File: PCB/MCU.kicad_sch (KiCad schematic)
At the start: 46 parts, among them J2 Conn_01x05_Pin, J3 Conn_01x02_Pin, SW1 SKRKAHE020, U1 STM32WLE5CCUx, U7 STM32WLE5C8Ux, Y1 ECS-TXO-25CSMV

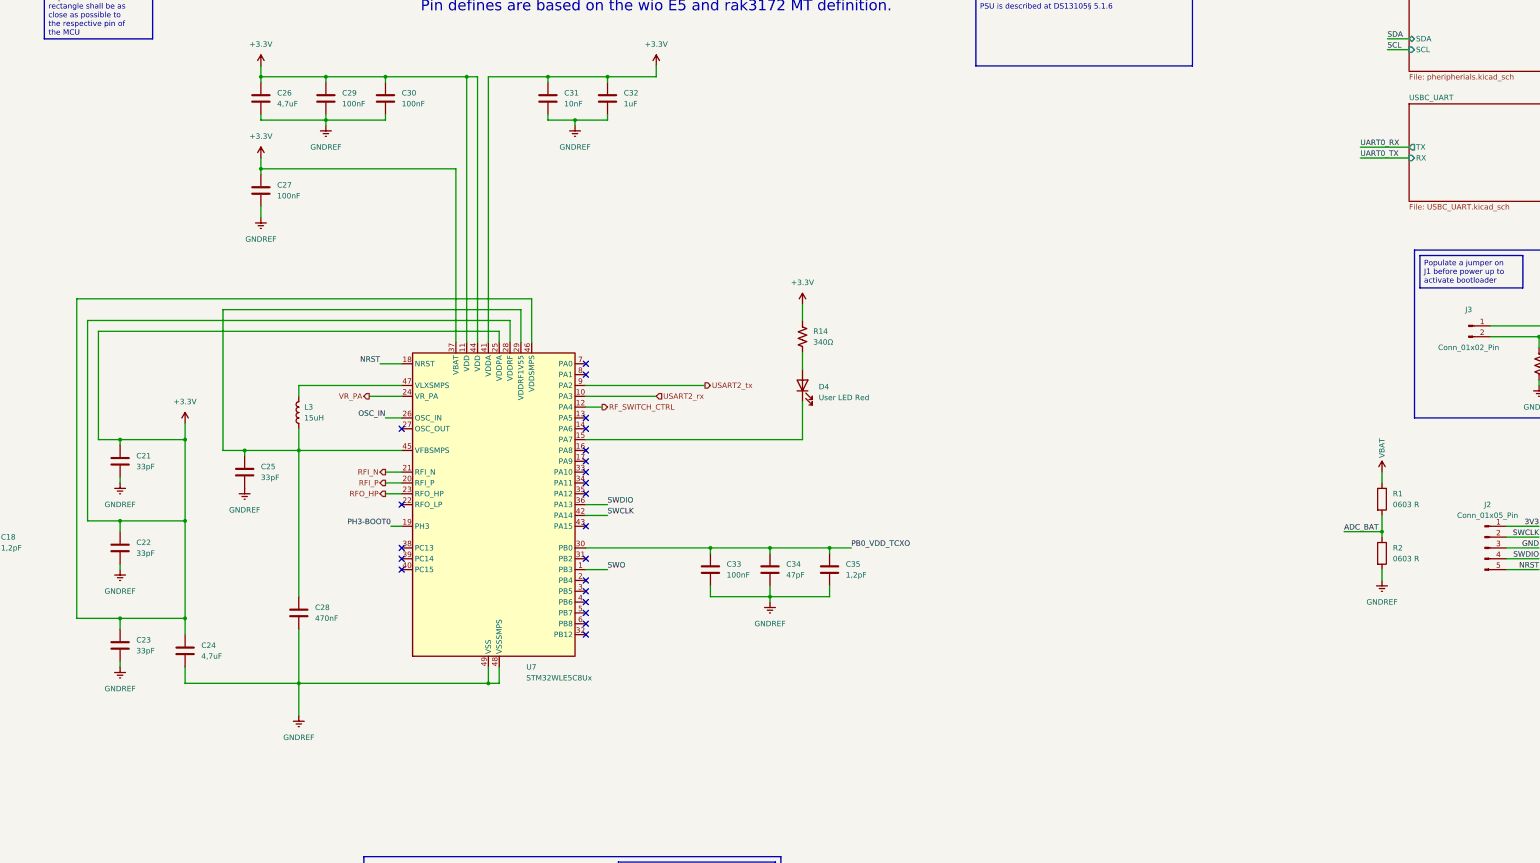
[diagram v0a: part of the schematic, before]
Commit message: finished the migration
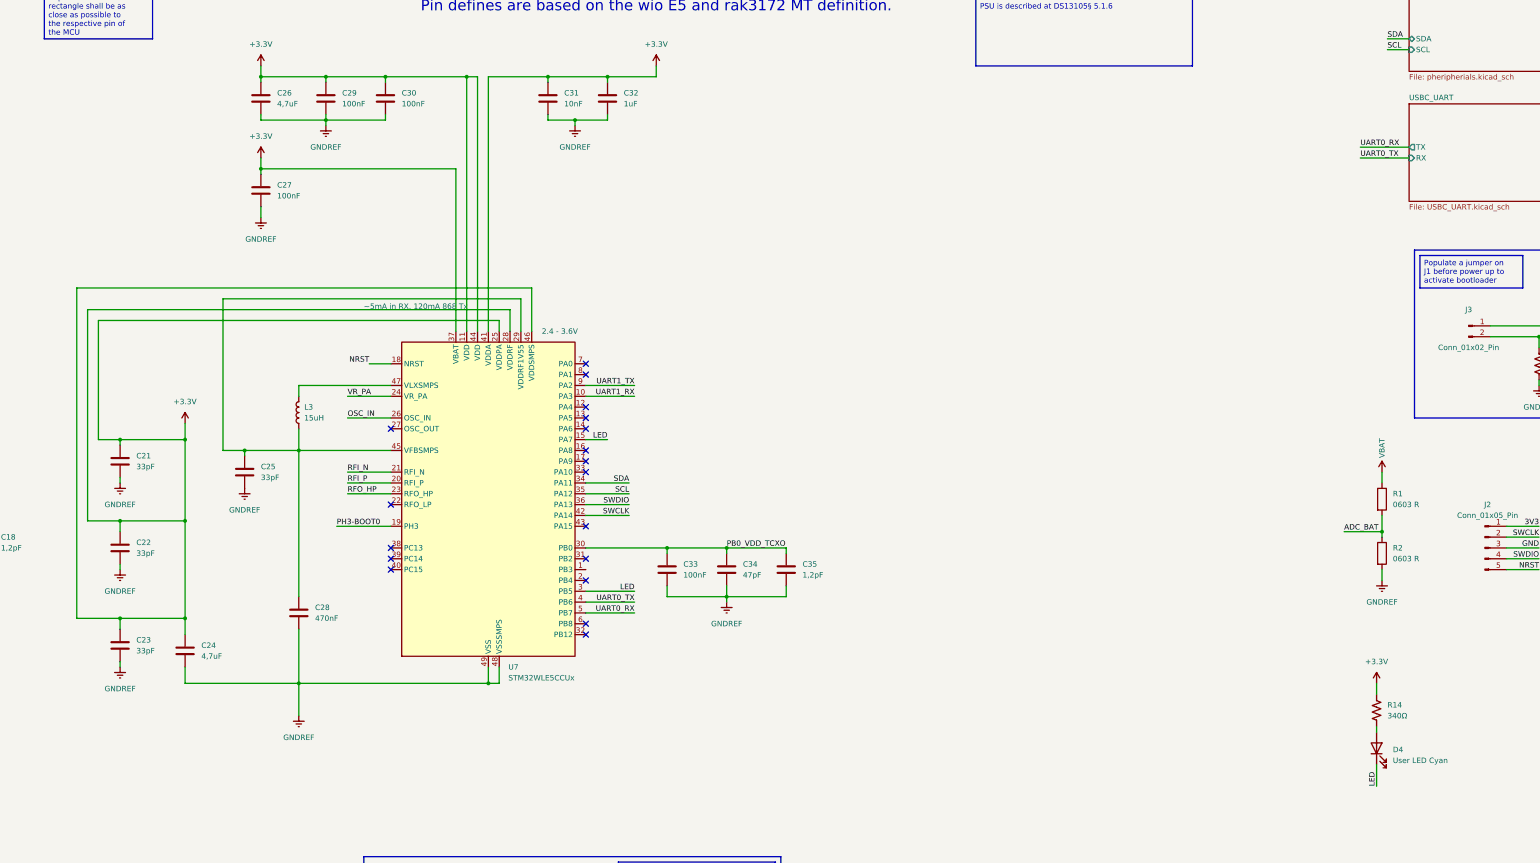
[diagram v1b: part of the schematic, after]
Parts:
- removed U7: STM32WLE5C8Ux, 100_QFN_package:QFN-48-1EP_7x7mm_P0.5mm_EP5.6x5.6mm_ThermalVias, symbol 100_MCU_ST_STM32WL:STM32WLE5C8Ux
- added U7: STM32WLE5CCUx, Package_DFN_QFN:QFN-48-1EP_7x7mm_P0.5mm_EP5.6x5.6mm, symbol MCU_ST_STM32WL:STM32WLE5CCUx
- D4: value User LED Red -> User LED Cyan; PartNumber B1811URO-20D000113U1930 -> (none)
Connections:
- net +3.3V: now also U7.11 (VDD), U7.25 (VDDPA), U7.28 (VDDRF), U7.37 (VBAT), U7.41 (VDDA), U7.44 (VDD), U7.46 (VDDSMPS)
- net GNDREF: now also U7.48 (VSSSMPS), U7.49 (VSS)
- net LED: now also D4.1 (K), U7.15 (PA7), U7.3 (PB5)
- net NRST: now also U7.18 (NRST)
- net OSC_IN: now also U7.26 (OSC_IN)
- net PB0_VDD_TCXO: now also U7.30 (PB0)
- net PH3-BOOT0: now also U7.19 (PH3)
- net RFI_N: now also U7.21 (RFI_N)
- net RFI_P: now also U7.20 (RFI_P)
- net RFO_HP: now also U7.23 (RFO_HP)
- net SCL: now also U7.35 (PA12)
- net SDA: now also U7.34 (PA11)
- net SWCLK: now also U7.42 (PA14)
- net SWDIO: now also U7.36 (PA13)
- net UART0_RX: now also U7.5 (PB7)
- net UART0_TX: now also U7.4 (PB6)
- net UART1_RX: now also U7.10 (PA3)
- net UART1_TX: now also U7.9 (PA2)
- net VR_PA: now also U7.24 (VR_PA)
- net at C25.2, C28.1, L3.1: now also U7.29 (VDDRF1V55), U7.45 (VFBSMPS)
- net at L3.2: now also U7.47 (VLXSMPS)
- no-connect marks 22 -> 18
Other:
- moved on the sheet: C33, C34, C35, D4, R14

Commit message: what about actually comiting
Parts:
- removed C10, C12: 0603 1uF, symbol Device:C
- removed C11, C6, C7: 0603 100nF, symbol Device:C
- removed C13, C8: 0603 4.7uF, symbol Device:C
- removed C16: 100nF, 1_capacitor_SMD:C_0402_1005Metric, symbol 0_generic_component:C
- removed C17: 47pF, 1_capacitor_SMD:C_0402_1005Metric, symbol 0_generic_component:C
- removed C18: 1,2pF, 1_capacitor_SMD:C_0402_1005Metric, symbol 0_generic_component:C
- removed C2: 0603 470nF, symbol Device:C
- removed C9: 0603 10nF, symbol Device:C
- removed D4: User LED Cyan, 3_LED_SMD:LED_0402_1005Metric, symbol 0_generic_component:LED
- removed L2: 15uH, symbol Device:L
- removed R1, R2: 0603 R, symbol Device:R
- removed R14: 340Ω, 0_resistor_SMD:R_0402_1005Metric, symbol 0_generic_component:R
- removed U1: STM32WLE5CCUx, Package_DFN_QFN:QFN-48-1EP_7x7mm_P0.5mm_EP5.6x5.6mm, symbol MCU_ST_STM32WL:STM32WLE5CCUx
- C1: value 0603 100nF -> 100nF; footprint Capacitor_SMD:C_0805_2012Metric_Pad1.18x1.45mm_HandSolder -> Resistor_SMD:R_0603_1608Metric_Pad0.98x0.95mm_HandSolder
- R3: value 0603 10K -> 10K; footprint Resistor_SMD:R_0805_2012Metric_Pad1.20x1.40mm_HandSolder -> Resistor_SMD:R_0603_1608Metric_Pad0.98x0.95mm_HandSolder
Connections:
- net +3V3 is gone; now on net +3.3V: R3.1
- net RF-switch_TX: now reaches U7.38 (PC13)
- net RF-switch_RX: now reaches U7.6 (PB8)
- no-connect marks 18 -> 16
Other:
- moved on the sheet: C1, C19, C20, C21, C22, C23, C24, C25, C26, C27, C28, C29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
